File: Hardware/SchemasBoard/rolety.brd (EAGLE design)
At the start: 47.9 x 22.9 mm, 30 parts, among them IC1 LNK304, IC2 MCP1703DB, K1 FRS1B, K2 FRS1B, T1 BC846, T2 BC846

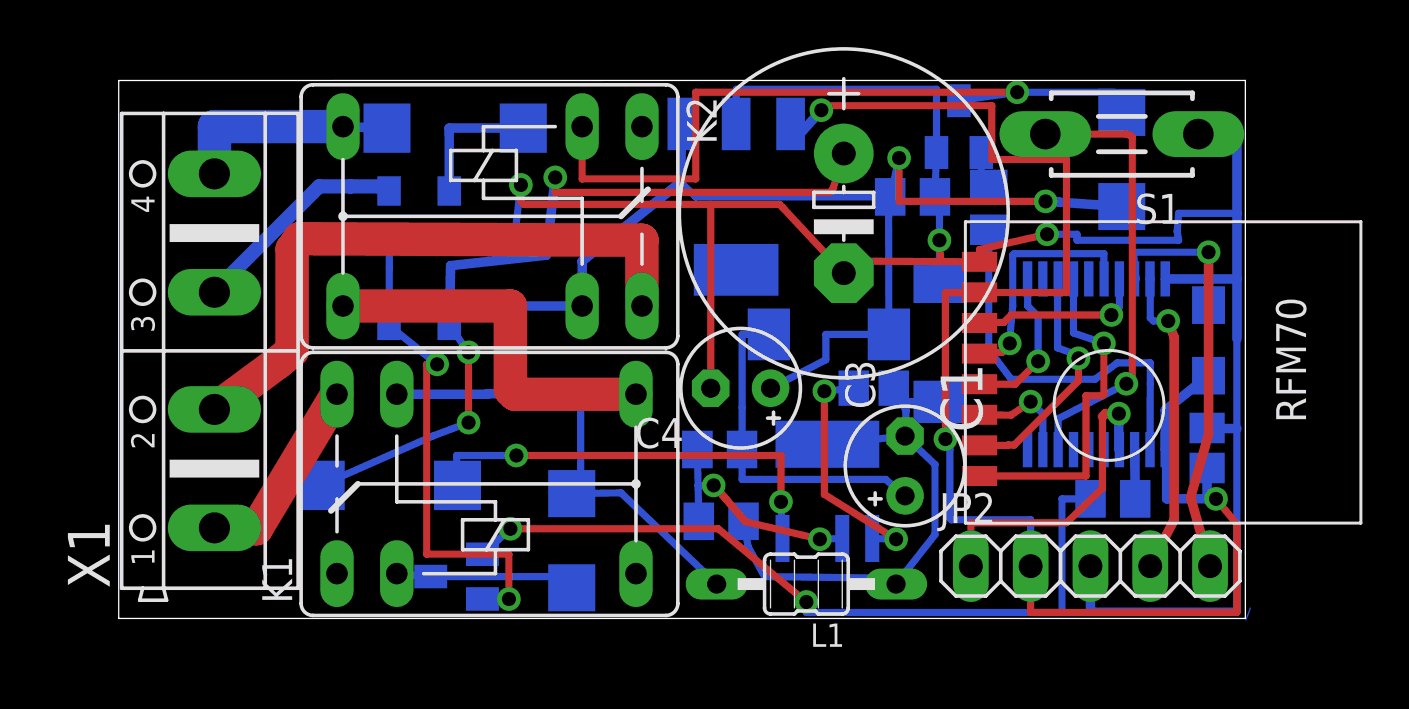
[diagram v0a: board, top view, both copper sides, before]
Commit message: a
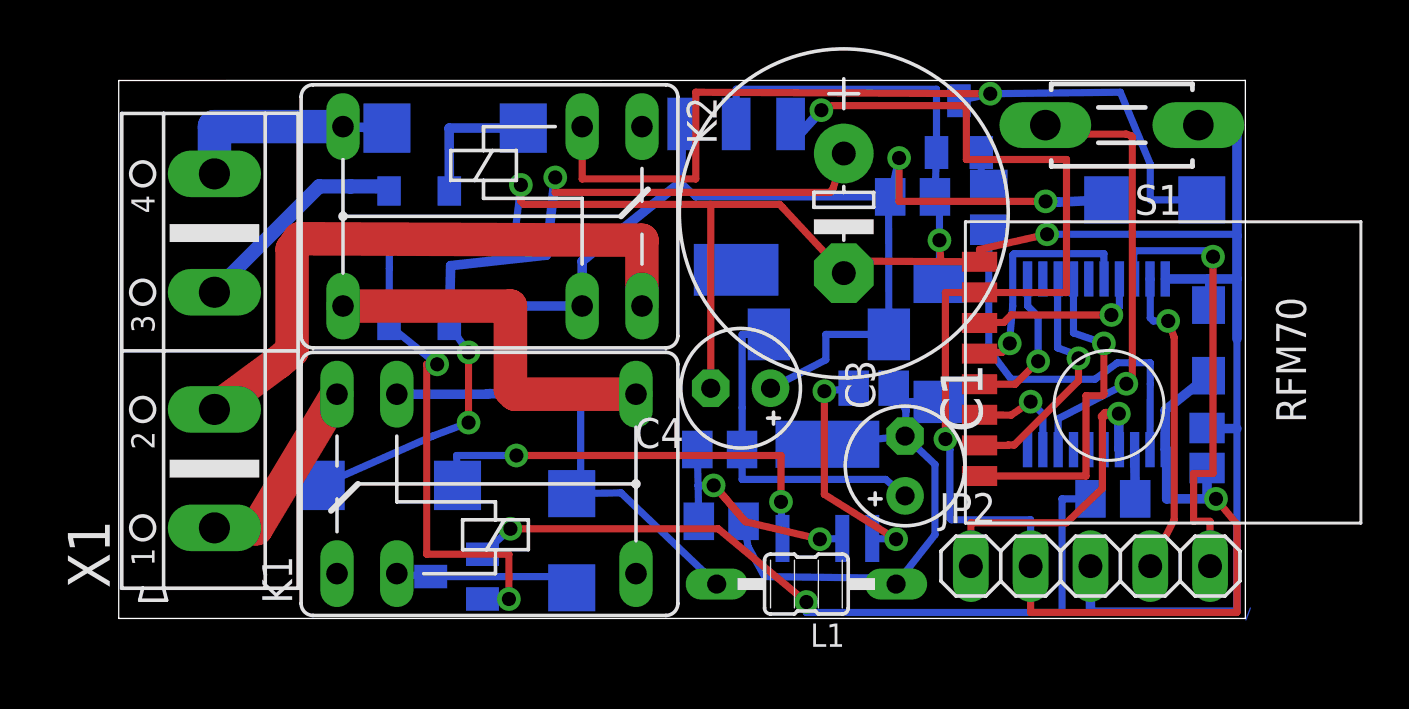
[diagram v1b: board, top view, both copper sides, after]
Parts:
- moved D2 2.21 mm to (42.9, 17.8), turned to 180 degrees
- moved S1 0.38 mm to (41.5, 21.0)
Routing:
- net N$24: track 31.9 -> 37.1 mm
- net N$19: track 17.9 -> 19.5 mm
- net GND: track 125.7 -> 124.4 mm
- net N$27: track 71.7 -> 71.1 mm
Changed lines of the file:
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@@
 <element name="D1" library="diode" package="SMA" value="MBRA340T3" x="18.0975" y="3.302" rot="MR270"/>
 <element name="C6" library="resistor" package="SMC_A" value="1uF" x="45.1485" y="11.811" rot="MR90"/>
-<element name="S1" library="switch-tact" package="DTS-3" value="DTS-3" x="41.4655" y="20.574" rot="R180"/>
+<element name="S1" library="switch-tact" package="DTS-3" value="DTS-3" x="41.4655" y="20.955" rot="R180"/>
 <element name="K2" library="relay" package="FRS1B" value="FRS1B" x="18.542" y="17.0815" rot="R180">
 <attribute name="OC_NEWARK" value="unknown" x="18.542" y="17.0815" size="1.778" layer="27" rot="R180" display="off"/>
@@
 </element>
 <element name="T2" library="transistor" package="SOT23" value="BC846" x="34.544" y="20.8915" rot="MR0"/>
-<element name="D2" library="diode" package="SMA" value="MBRA340T3" x="41.4655" y="19.4945" rot="MR90"/>
+<element name="D2" library="diode" package="SMA" value="MBRA340T3" x="42.8625" y="17.78" rot="MR180"/>
 <element name="R6" library="resistor" package="M2012" value="1 K" x="35.814" y="17.4625" rot="MR270"/>
 <element name="X1" library="con-ptr500" package="AK500/4" value="" x="2.921" y="11.3665" rot="R90">
@@
 <contactref element="S1" pad="1"/>
 <contactref element="T2" pad="2"/>
-<wire x1="44.7155" y1="20.574" x2="46.355" y2="20.574" width="0.4064" layer="16"/>
-<wire x1="46.355" y1="20.574" x2="46.355" y2="17.2085" width="0.4064" layer="16"/>
-<wire x1="46.355" y1="17.2085" x2="46.355" y2="14.42" width="0.4064" layer="16"/>
+<wire x1="44.7155" y1="20.955" x2="46.355" y2="20.574" width="0.4064" layer="16"/>
+<wire x1="46.355" y1="20.574" x2="46.355" y2="16.256" width="0.4064" layer="16"/>
+<wire x1="46.355" y1="16.256" x2="46.355" y2="14.42" width="0.4064" layer="16"/>
 <wire x1="46.355" y1="14.42" x2="46.355" y2="11.8745" width="0.4064" layer="16"/>
 <wire x1="43.311" y1="14.42" x2="45.1485" y2="14.42" width="0.4064" layer="16"/>
@@
 <wire x1="35.4205" y1="15.672" x2="38.2905" y2="16.3195" width="0.3048" layer="1"/>
 <via x="38.2905" y="16.3195" extent="1-16" drill="0.6"/>
-<wire x1="38.2905" y1="16.3195" x2="39.5605" y2="16.3195" width="0.3048" layer="16"/>
-<wire x1="39.5605" y1="16.3195" x2="39.5605" y2="16.0655" width="0.3048" layer="16"/>
-<wire x1="39.5605" y1="16.0655" x2="43.8785" y2="16.0655" width="0.3048" layer="16"/>
-<wire x1="43.8785" y1="16.0655" x2="43.815" y2="16.4465" width="0.3048" layer="16"/>
-<wire x1="43.815" y1="16.4465" x2="43.8785" y2="17.2085" width="0.3048" layer="16"/>
-<wire x1="43.8785" y1="17.2085" x2="46.355" y2="17.2085" width="0.3048" layer="16"/>
 <wire x1="45.1485" y1="13.311" x2="45.1485" y2="14.42" width="0.3048" layer="16"/>
 <wire x1="25.0825" y1="21.0058" x2="25.0825" y2="22.479" width="0.3048" layer="16"/>
@@
 <via x="33.7185" y="16.0655" extent="1-16" drill="0.6"/>
 <wire x1="33.7185" y1="16.0655" x2="33.779196875" y2="15.15824375" width="0.3048" layer="1"/>
+<wire x1="38.2905" y1="16.3195" x2="46.355" y2="16.3195" width="0.3048" layer="16"/>
+<wire x1="46.355" y1="16.3195" x2="46.355" y2="16.256" width="0.3048" layer="16"/>
 <wire x1="46.355" y1="0.3175" x2="46.736" y2="-0.0635" width="0" layer="19" extent="16-16"/>
 <wire x1="46.355" y1="11.8745" x2="46.355" y2="11.8505" width="0" layer="19" extent="16-16"/>
@@
 <via x="28.702" y="21.59" extent="1-16" drill="0.6"/>
 <wire x1="28.702" y1="21.59" x2="28.829" y2="21.7805" width="0.3048" layer="1"/>
-<wire x1="28.829" y1="21.7805" x2="35.941" y2="21.7805" width="0.3048" layer="1"/>
-<wire x1="35.941" y1="21.7805" x2="35.941" y2="19.4945" width="0.3048" layer="1"/>
-<wire x1="35.941" y1="19.4945" x2="39.116" y2="19.4945" width="0.3048" layer="1"/>
+<wire x1="28.829" y1="21.7805" x2="34.8615" y2="21.7805" width="0.3048" layer="1"/>
+<wire x1="34.8615" y1="21.7805" x2="34.8615" y2="19.4945" width="0.3048" layer="1"/>
+<wire x1="34.8615" y1="19.4945" x2="39.116" y2="19.4945" width="0.3048" layer="1"/>
 <wire x1="39.116" y1="19.4945" x2="39.116" y2="13.843" width="0.3048" layer="1"/>
 <wire x1="39.116" y1="13.843" x2="35.427" y2="13.843" width="0.3048" layer="1"/>
@@
 <contactref element="U$2" pad="19"/>
 <contactref element="JP2" pad="4"/>
-<wire x1="42.672" y1="2.2225" x2="43.688" y2="4.191" width="0.4064" layer="1"/>
-<wire x1="43.688" y1="4.191" x2="43.688" y2="11.938" width="0.4064" layer="1"/>
-<wire x1="43.688" y1="11.938" x2="43.434" y2="12.6365" width="0.4064" layer="1"/>
+<wire x1="42.672" y1="2.2225" x2="43.688" y2="4.191" width="0.3048" layer="1"/>
+<wire x1="43.688" y1="4.191" x2="43.688" y2="11.938" width="0.3048" layer="1"/>
+<wire x1="43.688" y1="11.938" x2="43.434" y2="12.6365" width="0.3048" layer="1"/>
 <via x="43.434" y="12.6365" extent="1-16" drill="0.6"/>
 <wire x1="43.434" y1="12.6365" x2="42.799" y2="12.6365" width="0.3048" layer="16"/>
@@
 <contactref element="U$2" pad="18"/>
 <contactref element="JP2" pad="5"/>
-<wire x1="45.212" y1="2.2225" x2="44.3865" y2="5.1435" width="0.4064" layer="1"/>
-<wire x1="44.3865" y1="5.1435" x2="45.1485" y2="7.8105" width="0.4064" layer="1"/>
-<wire x1="45.1485" y1="7.8105" x2="45.1485" y2="15.5575" width="0.4064" layer="1"/>
-<wire x1="45.1485" y1="15.5575" x2="44.1325" y2="16.1925" width="0" layer="19" extent="1-16"/>
-<wire x1="44.1325" y1="16.1925" x2="45.1485" y2="15.5575" width="0" layer="19" extent="1-16"/>
-<via x="45.1485" y="15.5575" extent="1-16" drill="0.6"/>
-<wire x1="45.1485" y1="15.5575" x2="41.9735" y2="15.5575" width="0.3048" layer="16"/>
-<wire x1="41.9735" y1="15.5575" x2="42.037" y2="14.446" width="0.3048" layer="16"/>
-<wire x1="42.037" y1="14.446" x2="42.011" y2="14.42" width="0.4064" layer="16"/>
+<wire x1="42.011" y1="14.42" x2="41.9735" y2="14.42" width="0.3048" layer="16"/>
+<wire x1="41.9735" y1="14.42" x2="41.9735" y2="15.621" width="0.3048" layer="16"/>
+<wire x1="41.9735" y1="15.621" x2="45.339" y2="15.621" width="0.3048" layer="16"/>
+<wire x1="45.339" y1="15.621" x2="45.339" y2="15.367" width="0.3048" layer="16"/>
+<via x="45.339" y="15.367" extent="1-16" drill="0.6"/>
+<wire x1="45.339" y1="15.367" x2="45.339" y2="6.1595" width="0.3048" layer="1"/>
+<wire x1="45.339" y1="6.1595" x2="44.5135" y2="6.1595" width="0.3048" layer="1"/>
+<wire x1="44.5135" y1="6.1595" x2="44.5135" y2="4.1275" width="0.3048" layer="1"/>
+<wire x1="44.5135" y1="4.1275" x2="45.212" y2="4.1275" width="0.3048" layer="1"/>
+<wire x1="45.212" y1="4.1275" x2="45.212" y2="2.2225" width="0.3048" layer="1"/>
 </signal>
 <signal name="N$15">
@@
 <wire x1="41.8465" y1="20.5105" x2="41.656" y2="20.574" width="0.3048" layer="1"/>
 <wire x1="41.656" y1="20.574" x2="38.7985" y2="20.574" width="0.3048" layer="1"/>
-<wire x1="38.7985" y1="20.574" x2="38.2155" y2="20.574" width="0.4064" layer="1"/>
+<wire x1="38.7985" y1="20.574" x2="38.2155" y2="20.955" width="0.4064" layer="1"/>
 </signal>
 <signal name="N$7">
@@
 <contactref element="K2" pad="2"/>
 <contactref element="T2" pad="3"/>
-<wire x1="41.4655" y1="21.4945" x2="41.148" y2="22.352" width="0.3048" layer="16"/>
-<wire x1="41.148" y1="22.352" x2="37.0205" y2="22.352" width="0.3048" layer="16"/>
-<via x="37.0205" y="22.352" extent="1-16" drill="0.6"/>
-<wire x1="37.0205" y1="22.352" x2="23.368" y2="22.352" width="0.3048" layer="1"/>
+<wire x1="44.8625" y1="17.78" x2="42.672" y2="17.78" width="0.3048" layer="16"/>
+<wire x1="42.672" y1="17.78" x2="42.672" y2="19.304" width="0.3048" layer="16"/>
+<wire x1="42.672" y1="19.304" x2="41.402" y2="22.352" width="0.3048" layer="16"/>
+<wire x1="41.402" y1="22.352" x2="35.8775" y2="22.2885" width="0.3048" layer="16"/>
+<via x="35.8775" y="22.2885" extent="1-16" drill="0.6"/>
+<wire x1="35.8775" y1="22.2885" x2="23.368" y2="22.352" width="0.3048" layer="1"/>
 <wire x1="23.368" y1="22.352" x2="23.368" y2="18.669" width="0.3048" layer="1"/>
 <wire x1="23.368" y1="18.669" x2="18.542" y2="18.669" width="0.3048" layer="1"/>
 <wire x1="18.542" y1="18.669" x2="18.542" y2="20.8915" width="0.3048" layer="1"/>
-<wire x1="34.544" y1="21.9915" x2="37.0205" y2="22.352" width="0.3048" layer="16"/>
+<wire x1="34.544" y1="21.9915" x2="35.8775" y2="22.2885" width="0.3048" layer="16"/>
 </signal>
 <signal name="N$27">
@@
 <wire x1="22.7203" y1="18.5293" x2="18.542" y2="15.1765" width="0.4064" layer="16"/>
 <wire x1="18.542" y1="15.1765" x2="18.542" y2="13.2715" width="0.4064" layer="16"/>
-<wire x1="41.4655" y1="17.4945" x2="38.7665" y2="17.685" width="0.4064" layer="16"/>
+<wire x1="40.8625" y1="17.78" x2="38.7665" y2="17.685" width="0.4064" layer="16"/>
 <wire x1="38.7665" y1="17.685" x2="38.227" y2="17.7165" width="0.4064" layer="16"/>
 <via x="38.227" y="17.7165" extent="1-16" drill="0.6"/>

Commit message: aaa
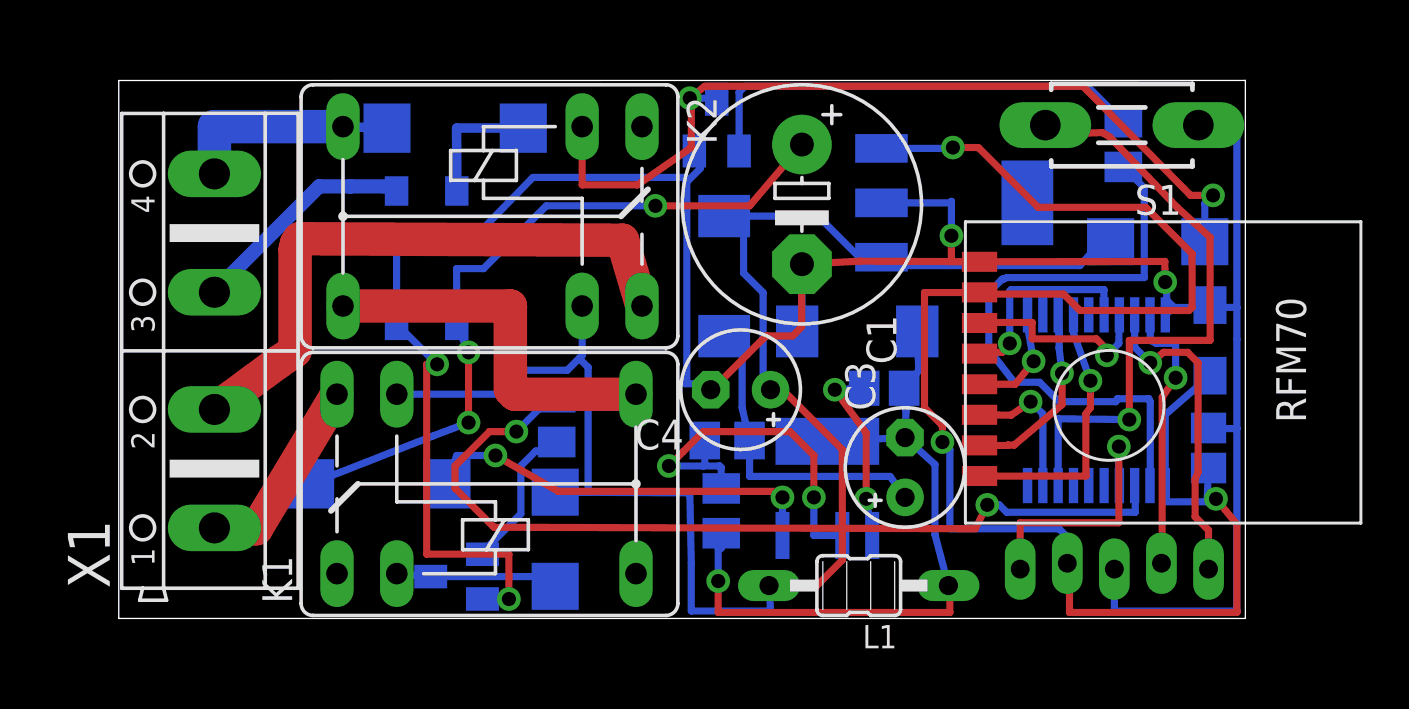
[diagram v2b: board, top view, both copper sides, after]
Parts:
- removed JP2: (no value), pinhead:1X05
- removed R7: 2 K, resistor:M2012
- added U$3: PROGRAMMINGHEADERDIP, rfm70:PROGHEADER
- C1: device resistor:E5-13 -> resistor:E5-10,5
- moved R5 23.9 mm to (17.5, 8.45), turned to 90 degrees
- moved T2 10.3 mm to (24.3, 21.0)
- moved IC2 9.27 mm to (34.4, 17.7), turned to 90 degrees
- moved R6 6.31 mm to (41.5, 20.1)
- moved D4 5.09 mm to (24.6, 14.5), turned to 90 degrees
- moved D3 3.52 mm to (30.2, 12.2), turned to 0 degrees
- moved L1 2.22 mm to (30.3, 1.40)
- moved C1 1.82 mm to (27.9, 17.6)
- moved D2 1.78 mm to (43.0, 16.0)
- moved U$2 1.52 mm to (40.4, 9.27)
- moved D1 0.70 mm to (17.4, 3.37)
- moved R3 0.50 mm to (24.7, 7.56)
- moved R1 0.45 mm to (9.91, 5.71)
- moved C2 0.44 mm to (31.4, 9.78)
- moved R4 0.44 mm to (24.4, 4.57), turned to 270 degrees
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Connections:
- net GND: now also U$3.GND; no longer JP2.3, R7.1
- net N$17: now also U$3.VDD; no longer JP2.2
- net N$18: now also U$3.PGD; no longer JP2.4
- net N$19: now also U$3.PGC; no longer JP2.5
- net N$25: now also U$3.MCLR; no longer JP2.1
- net N$27: no longer R7.2
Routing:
- net N$35: track 2.09 -> 38.3 mm, vias 0 -> 2
- net N$15: track 32.6 -> 6.37 mm, vias 2 -> 0
- net N$28: track 1.64 -> 19.6 mm
- net GND: track 124.4 -> 114.6 mm, vias 5 -> 4
- net N$6: track 16.5 -> 25.9 mm
- net N$13: track 22.8 -> 29.8 mm, vias 0 -> 1
- net N$5: track 19.2 -> 26.0 mm
- net N$19: track 19.5 -> 13.7 mm
- net N$2: track 35.2 -> 30.8 mm
- net N$11: track 12.0 -> 16.0 mm
- net N$21: track 14.5 -> 11.6 mm
- net N$17: track 66.6 -> 69.4 mm
- net N$10: track 10.2 -> 7.89 mm
- net N$12: track 10.2 -> 7.96 mm
- net N$25: track 13.4 -> 11.1 mm
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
